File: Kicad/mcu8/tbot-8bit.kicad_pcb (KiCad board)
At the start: 2 copper layers, 80 x 100 mm, 90 parts, among them IC101 TI-TLV1117-50-SOT, IC201 PIC16F1778, IC301 MICROCHIP-MCP2221A-ISL, K101 Battery, K201 MCU 1, K202 ICSP, K203 MCU 2, K301 FRONT #1, K302 FRONT #2, K303 VIN, K304 +5V, K305 FRONT #3, K306 SERVO LEFT, K307 LEFT, K308 USB/UART, K309 SERVO RIGHT, K310 RIGHT, Q101 DIODESINC-DMP2305U-SOT-23, Q102 DIODESINC-DMP2305U-SOT-23

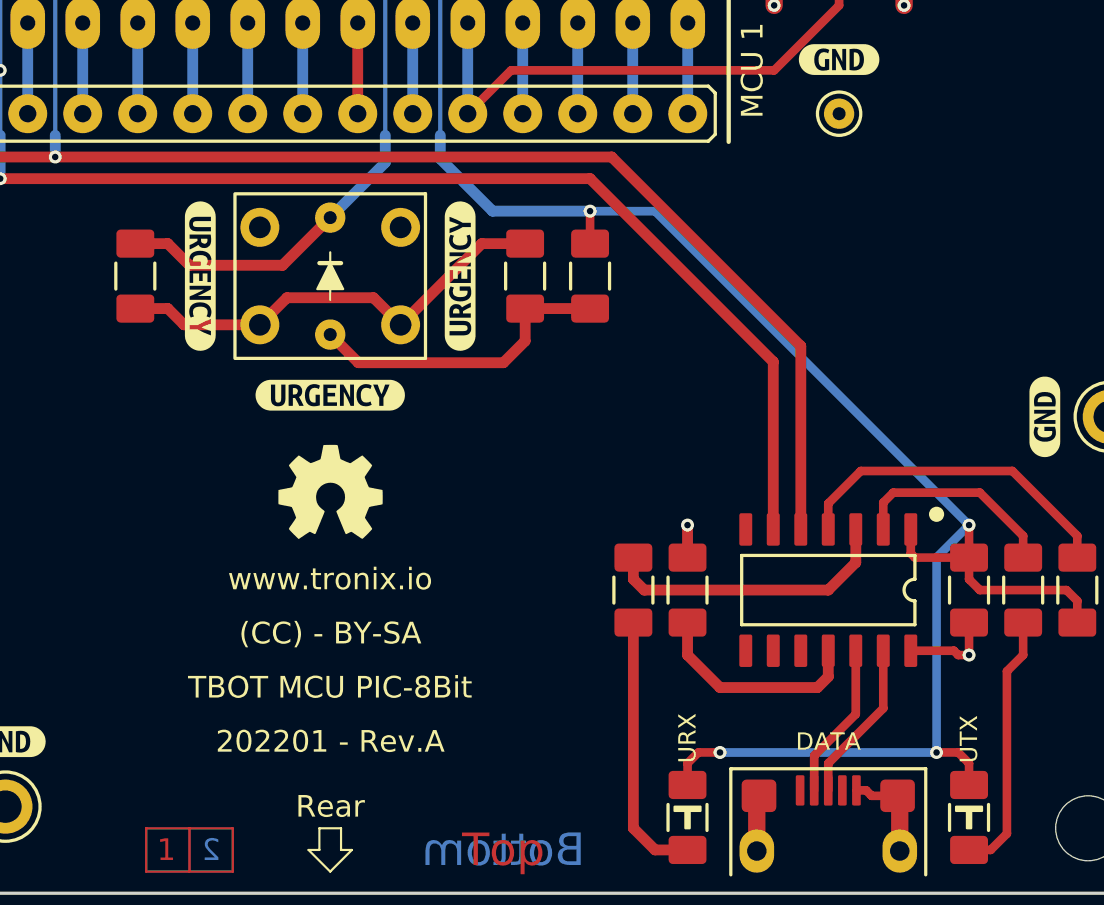
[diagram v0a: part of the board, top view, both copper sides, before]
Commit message: Update
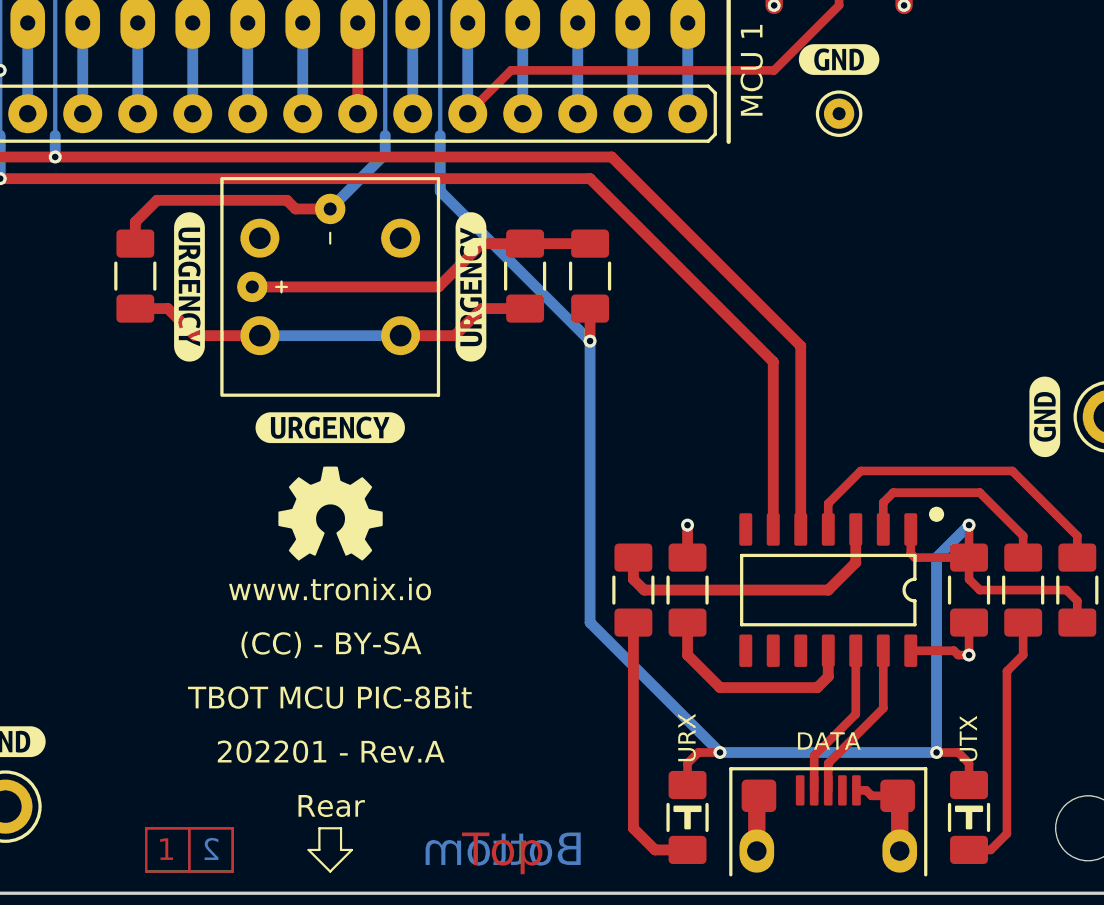
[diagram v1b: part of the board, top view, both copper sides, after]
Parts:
- S301: value EMERGENCY -> URGENCY; footprint tronixio:E-SWITCH-TL1240XQ1JXXX -> tronixio:zzzOMRON-B3W9000-X1
- moved kibuzzard-627FC6B4 1.50 mm to (140.0, 128.5)
- moved G*** 1.00 mm to (140.0, 132.5) (x2)
- moved kibuzzard-627FC6B4 0.71 mm to (146.5, 122.0)
- moved kibuzzard-627FC6B4 0.71 mm to (133.5, 122.0)
- moved S301 0.50 mm to (140.0, 122.0), turned to 90 degrees
- turned R301 to -90 degrees
- turned R302 to 90 degrees
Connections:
- net /HID/RB0/EMERGENCY renamed /HID/RB0/URGENCY
- S301 pad 1: GND -> Net-(R302-Pad1)
- S301 pad 2: GND -> Net-(R302-Pad1)
- S301 pad 3: Net-(R302-Pad1) -> GND
- S301 pad 4: Net-(R302-Pad1) -> GND
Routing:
- net Net-(R301-Pad1): track 14.5 -> 16.4 mm
- net Net-(R302-Pad1): track 20.9 -> 19.0 mm
- net +5V: track 308.7 -> 310.0 mm
